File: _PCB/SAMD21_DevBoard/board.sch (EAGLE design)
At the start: 1 part, among them U1 ATSAMD21G-A

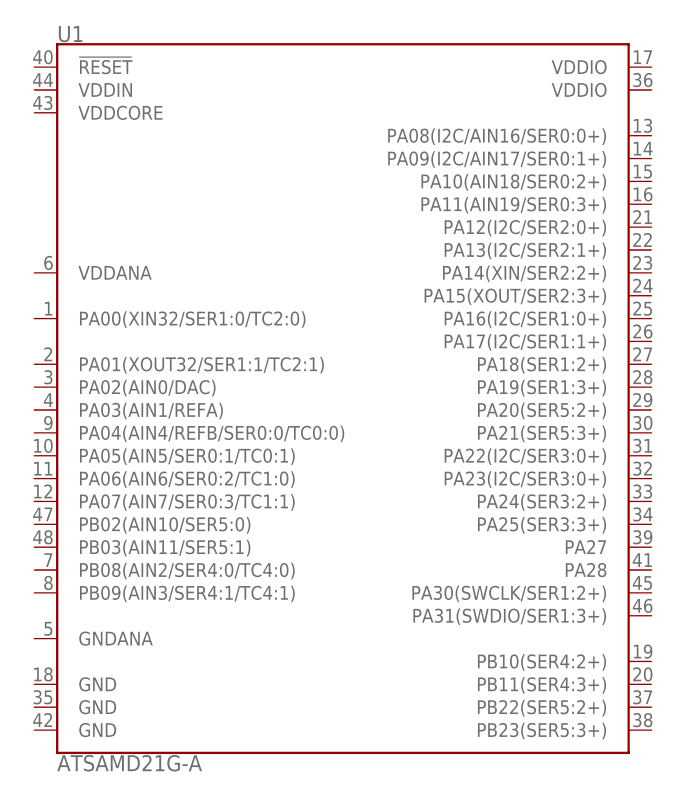
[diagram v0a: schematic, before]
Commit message: added samples
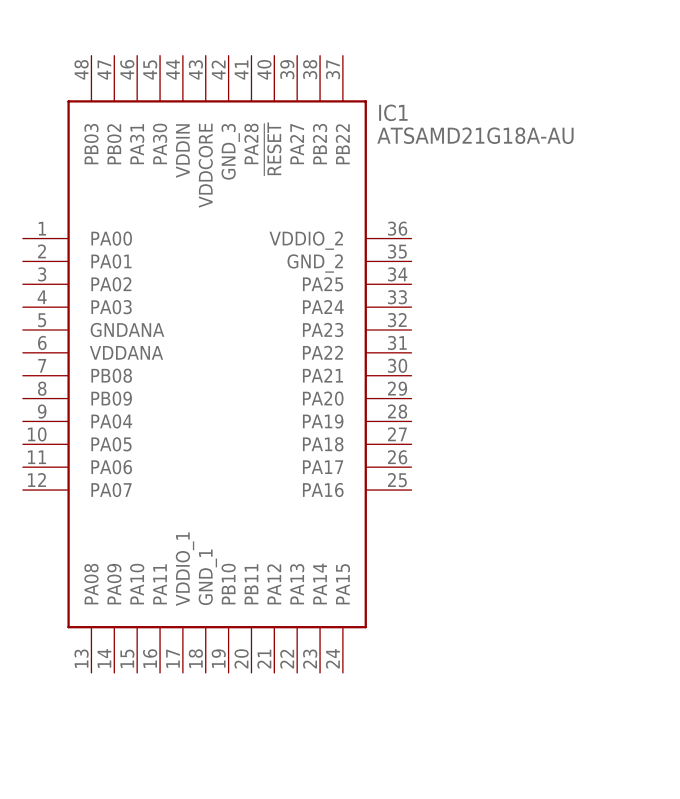
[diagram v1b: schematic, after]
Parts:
- removed U1: ATSAMD21G-A, SparkFun-IC-Microcontroller:ATSAMD21G-A
- added IC1: ATSAMD21G18A-AU, SamacSys_Parts:ATSAMD21G18A-AU
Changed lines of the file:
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@@
 <parts>
 <part name="FRAME1" library="frames" library_urn="urn:adsk.eagle:library:229" deviceset="A4L-LOC" device=""/>
-<part name="U1" library="SparkFun-IC-Microcontroller" library_urn="urn:adsk.eagle:library:525" deviceset="ATSAMD21G" device="-A" package3d_urn="urn:adsk.eagle:package:38963/1"/>
+<part name="IC1" library="SamacSys_Parts" deviceset="ATSAMD21G18A-AU" device=""/>
 </parts>
 <sheets>
@@
 <attribute name="SHEET" x="230.505" y="5.08" size="2.54" layer="94"/>
 </instance>
-<instance part="U1" gate="G$1" x="116.84" y="91.44" smashed="yes">
-<attribute name="NAME" x="86.36" y="137.414" size="1.778" layer="95"/>
-<attribute name="VALUE" x="86.36" y="58.166" size="1.778" layer="96" align="top-left"/>
+<instance part="IC1" gate="G$1" x="104.14" y="101.6" smashed="yes">
+<attribute name="NAME" x="121.92" y="129.54" size="1.778" layer="95" align="center-left"/>
+<attribute name="VALUE" x="121.92" y="127" size="1.778" layer="96" align="center-left"/>
 </instance>
 </instances>
@@
 will not be understood (or retained) with this version.
 </note>
-<note version="8.3" severity="warning">
-Since Version 8.3, EAGLE supports the association of 3D packages
-with devices in libraries, schematics, and board files. Those 3D
-packages will not be understood (or retained) with this version.
-</note>
 </compatibility>
